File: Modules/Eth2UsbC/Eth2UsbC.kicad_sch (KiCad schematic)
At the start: 1 part, among them U1 RTL8153B-VB-CG

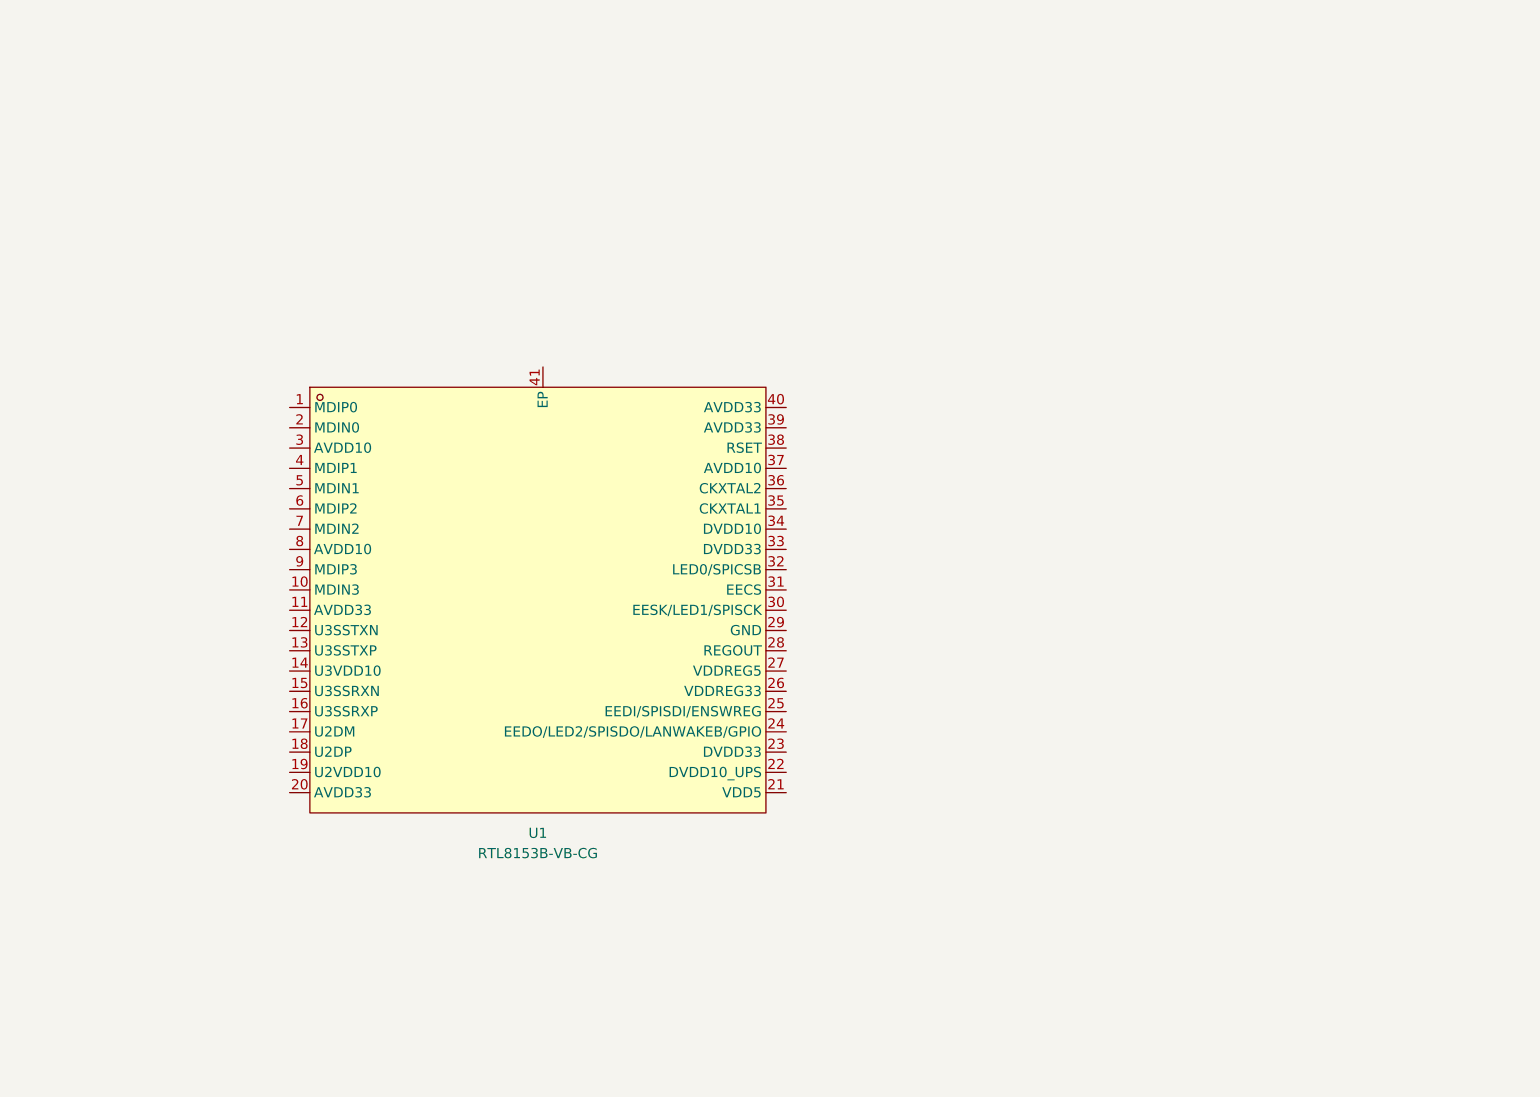
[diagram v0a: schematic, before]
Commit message: some changes
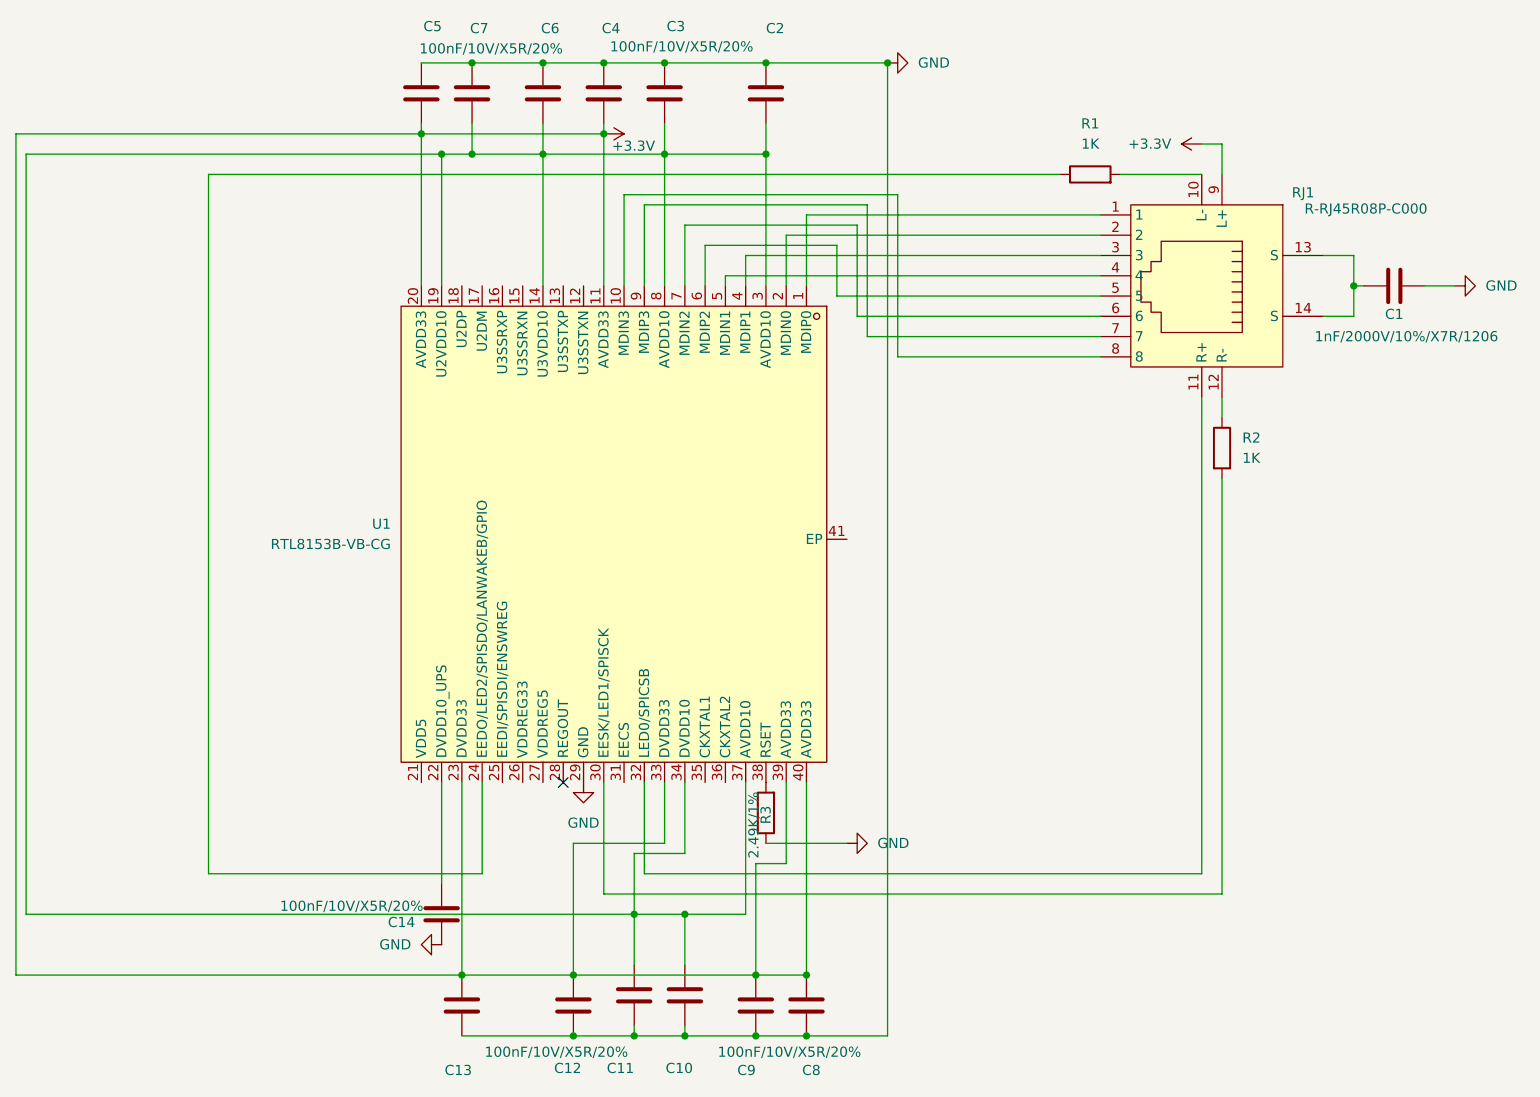
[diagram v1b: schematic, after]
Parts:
- added C1: 1nF/2000V/10%/X7R/1206, symbol Device:C
- added C10, C11, C12, C13, C14, C2, C3, C4, C5, C6, C7, C8, C9: 100nF/10V/X5R/20%, symbol Device:C
- added R1, R2: 1K, symbol Device:R
- added R3: 2.49K/1%, symbol Device:R
- added RJ1: R-RJ45R08P-C000, easyeda2kicad:RJ45-TH_R-RJ45R08P-C000, symbol C386757:R-RJ45R08P-C000
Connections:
- net at U1.1 (MDIP0): now also RJ1.1
- net at U1.10 (MDIN3): now also RJ1.8
- net +3.3V: now reaches U1.11 (AVDD33)
- net +3.3V: now also U1.20 (AVDD33), U1.23 (DVDD33), U1.33 (DVDD33), U1.39 (AVDD33), U1.40 (AVDD33), C12.2, C13.2, C4.2, C5.2, C8.2, C9.2, RJ1.9 (L+)
- net at U1.14 (U3VDD10): now also U1.19 (U2VDD10), U1.3 (AVDD10), U1.34 (DVDD10), U1.37 (AVDD10), U1.8 (AVDD10), C10.2, C11.2, C2.2, C3.2, C6.2, C7.2
- net at U1.2 (MDIN0): now also RJ1.2
- net at U1.22 (DVDD10_UPS): now also C14.2
- net at U1.24 (EEDO/LED2/SPISDO/LANWAKEB/GPIO): now also R1.1
- net GND: now reaches U1.29 (GND)
- net GND: now also C1.2, C10.1, C11.1, C12.1, C13.1, C14.1, C2.1, C3.1, C4.1, C5.1, C6.1, C7.1, C8.1, C9.1, R3.1
- net at U1.30 (EESK/LED1/SPISCK): now also R2.2
- net at U1.32 (LED0/SPICSB): now also RJ1.11 (R+)
- net at U1.38 (RSET): now also R3.2
- net at U1.4 (MDIP1): now also RJ1.3
- net at U1.5 (MDIN1): now also RJ1.4
- net at U1.6 (MDIP2): now also RJ1.5
- net at U1.7 (MDIN2): now also RJ1.6
- net at U1.9 (MDIP3): now also RJ1.7
- new net: R2.1, RJ1.12 (R-)
- new net: C1.1, RJ1.13 (S), RJ1.14 (S)
- new net: R1.2, RJ1.10 (L-)
- no-connect marks 0 -> 1
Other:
- moved on the sheet: U1
